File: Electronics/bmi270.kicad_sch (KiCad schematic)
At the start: 3 parts

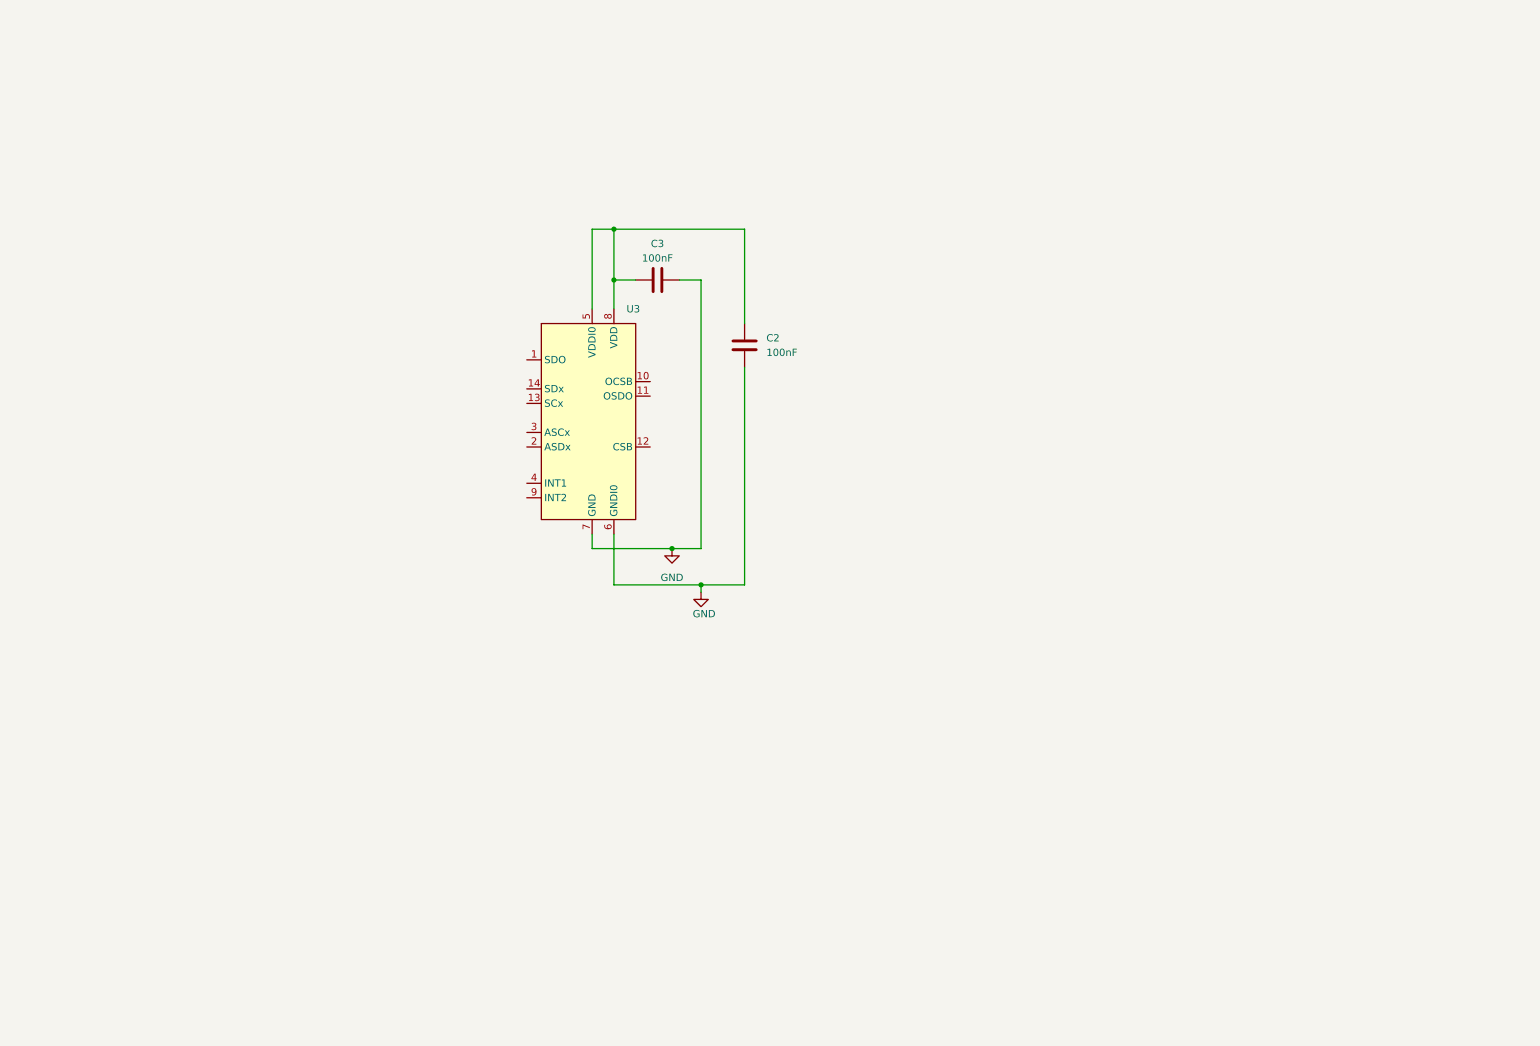
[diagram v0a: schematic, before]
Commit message: gyros done
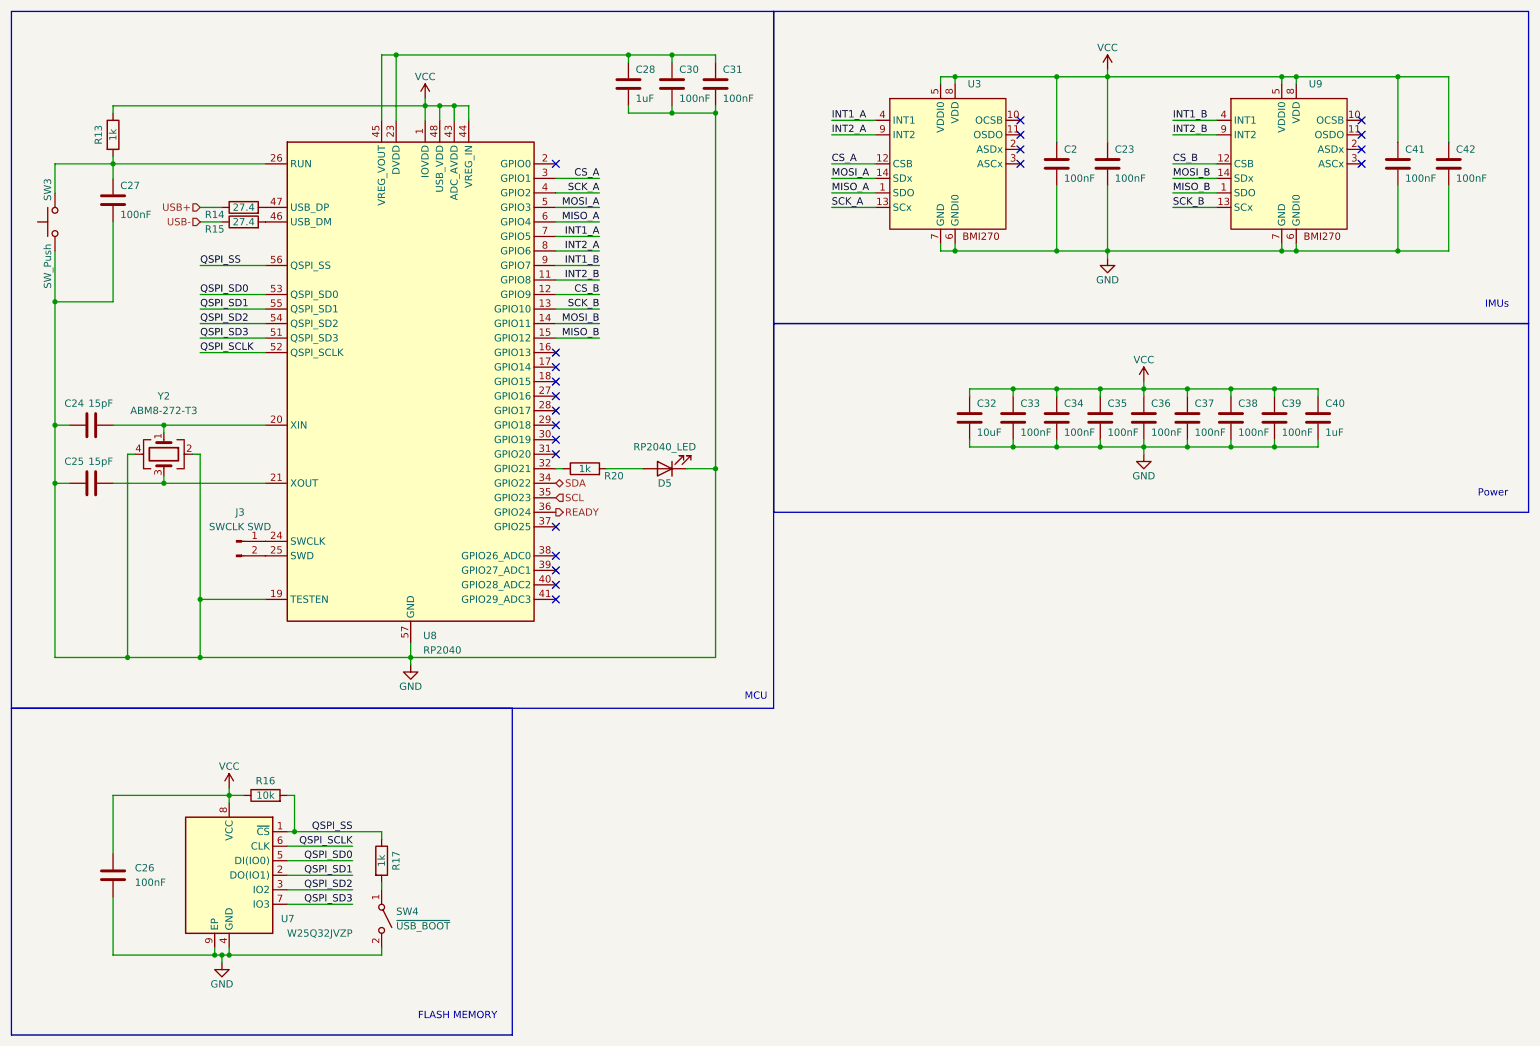
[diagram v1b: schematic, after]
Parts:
- removed C3: 100nF, symbol Device:C
- added C23, C26, C27, C30, C31, C33, C34, C35, C36, C37, C38, C39, C41, C42: 100nF, symbol Device:C
- added C24, C25: 15pF, symbol Device:C
- added C28, C40: 1uF, symbol Device:C
- added C32: 10uF, symbol Device:C
- added D5: RP2040_LED, symbol Device:LED
- added J3: SWCLK SWD, symbol Connector:Conn_01x02_Pin
- added R13, R17, R20: 1k, symbol Device:R
- added R14, R15: 27.4, symbol Device:R
- added R16: 10k, symbol Device:R
- added SW3: SW_Push, symbol Switch:SW_Push
- added SW4: ~{USB_BOOT}, symbol Switch:SW_SPST
- added U7: W25Q32JVZP, Package_SON:WSON-8-1EP_6x5mm_P1.27mm_EP3.4x4.3mm, symbol Memory_Flash:W25Q32JVZP
- added U8: RP2040, Package_DFN_QFN:QFN-56-1EP_7x7mm_P0.4mm_EP3.2x3.2mm, symbol MCU_RaspberryPi:RP2040
- added U9: ~, Package_LGA:Bosch_LGA-14_3x2.5mm_P0.5mm, symbol BMI270:BMI270
- added Y2: ABM8-272-T3, symbol Device:Crystal_GND24
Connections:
- net GND: now also C23.2, C24.1, C25.1, C26.2, C27.2, C28.2, C30.2, C31.2, C32.2, C33.2, C34.2, C35.2, C36.2, C37.2, C38.2, C39.2, C40.2, C41.2, C42.2, D5.1 (K), SW3.1, SW4.2 (B), U7.4 (GND), U7.9 (EP), U8.19 (TESTEN), U8.57 (GND), U9.6 (GNDI0), U9.7 (GND), Y2.2, Y2.4
- net VCC: now reaches C2.1, U3.5 (VDDI0), U3.8 (VDD)
- net VCC: now also C23.1, C26.1, C32.1, C33.1, C34.1, C35.1, C36.1, C37.1, C38.1, C39.1, C40.1, C41.1, C42.1, R13.1, R16.1, U7.8 (VCC), U8.1 (IOVDD), U8.10 (IOVDD), U8.22 (IOVDD), U8.33 (IOVDD), U8.42 (IOVDD), U8.43 (ADC_AVDD), U8.44 (VREG_IN), U8.48 (USB_VDD), U8.49 (IOVDD), U9.5 (VDDI0), U9.8 (VDD)
- net MISO_A: now reaches U3.1 (SDO)
- net MISO_A: now also U8.6 (GPIO4)
- net CS_A: now reaches U3.12 (CSB)
- net CS_A: now also U8.3 (GPIO1)
- net SCK_A: now reaches U3.13 (SCx)
- net SCK_A: now also U8.4 (GPIO2)
- net MOSI_A: now reaches U3.14 (SDx)
- net MOSI_A: now also U8.5 (GPIO3)
- net INT1_A: now reaches U3.4 (INT1)
- net INT1_A: now also U8.7 (GPIO5)
- net INT2_A: now reaches U3.9 (INT2)
- net INT2_A: now also U8.8 (GPIO6)
- new net: C28.1, C30.1, C31.1, U8.23 (DVDD), U8.45 (VREG_VOUT), U8.50 (DVDD)
- new net: C27.1, R13.2, SW3.2, U8.26 (RUN)
- new net: J3.1 (Pin_1), U8.24 (SWCLK)
- new net: J3.2 (Pin_2), U8.25 (SWD)
- new net: C24.2, U8.20 (XIN), Y2.1
- new net: C25.2, U8.21 (XOUT), Y2.3
- new net: R20.1, U8.32 (GPIO21)
- new net: R15.2, U8.46 (USB_DM)
- new net: R14.2, U8.47 (USB_DP)
- new net: D5.2 (A), R20.2
- new net: R17.2, SW4.1 (A)
- new net CS_B: U8.12 (GPIO9), U9.12 (CSB)
- new net INT1_B: U8.9 (GPIO7), U9.4 (INT1)
- new net INT2_B: U8.11 (GPIO8), U9.9 (INT2)
- new net MISO_B: U8.15 (GPIO12), U9.1 (SDO)
- new net MOSI_B: U8.14 (GPIO11), U9.14 (SDx)
- new net QSPI_SCLK: U7.6 (CLK), U8.52 (QSPI_SCLK)
- new net QSPI_SD0: U7.5 (DI(IO0)), U8.53 (QSPI_SD0)
- new net QSPI_SD1: U7.2 (DO(IO1)), U8.55 (QSPI_SD1)
- new net QSPI_SD2: U7.3 (IO2), U8.54 (QSPI_SD2)
- new net QSPI_SD3: U7.7 (IO3), U8.51 (QSPI_SD3)
- new net QSPI_SS: R16.2, R17.1, U7.1 (~{CS}), U8.56 (QSPI_SS)
- new net READY: U8.36 (GPIO24)
- new net SCK_B: U8.13 (GPIO10), U9.13 (SCx)
- new net SCL: U8.35 (GPIO23)
- new net SDA: U8.34 (GPIO22)
- new net USB+: R14.1
- new net USB-: R15.1
- no-connect marks 0 -> 22
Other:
- note added: "FLASH MEMORY"
- note added: "IMUs"
- note added: "MCU"
- note added: "Power"
